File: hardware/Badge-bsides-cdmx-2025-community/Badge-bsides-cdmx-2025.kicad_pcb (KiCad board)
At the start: 2 copper layers, 50 x 110 mm, 30 parts, among them J1 SWDIO, J3 ADDON, J4 Conn_01x04_Pin, J5 I2C, J6 Conn_01x04_Pin, P6 USB_C_Plug_USB2.0, Q3 DMG3415U-7, SW11 ON, SW2 RESET, U1 PY32F030F28U6TR, U6 AP2112K-3.3

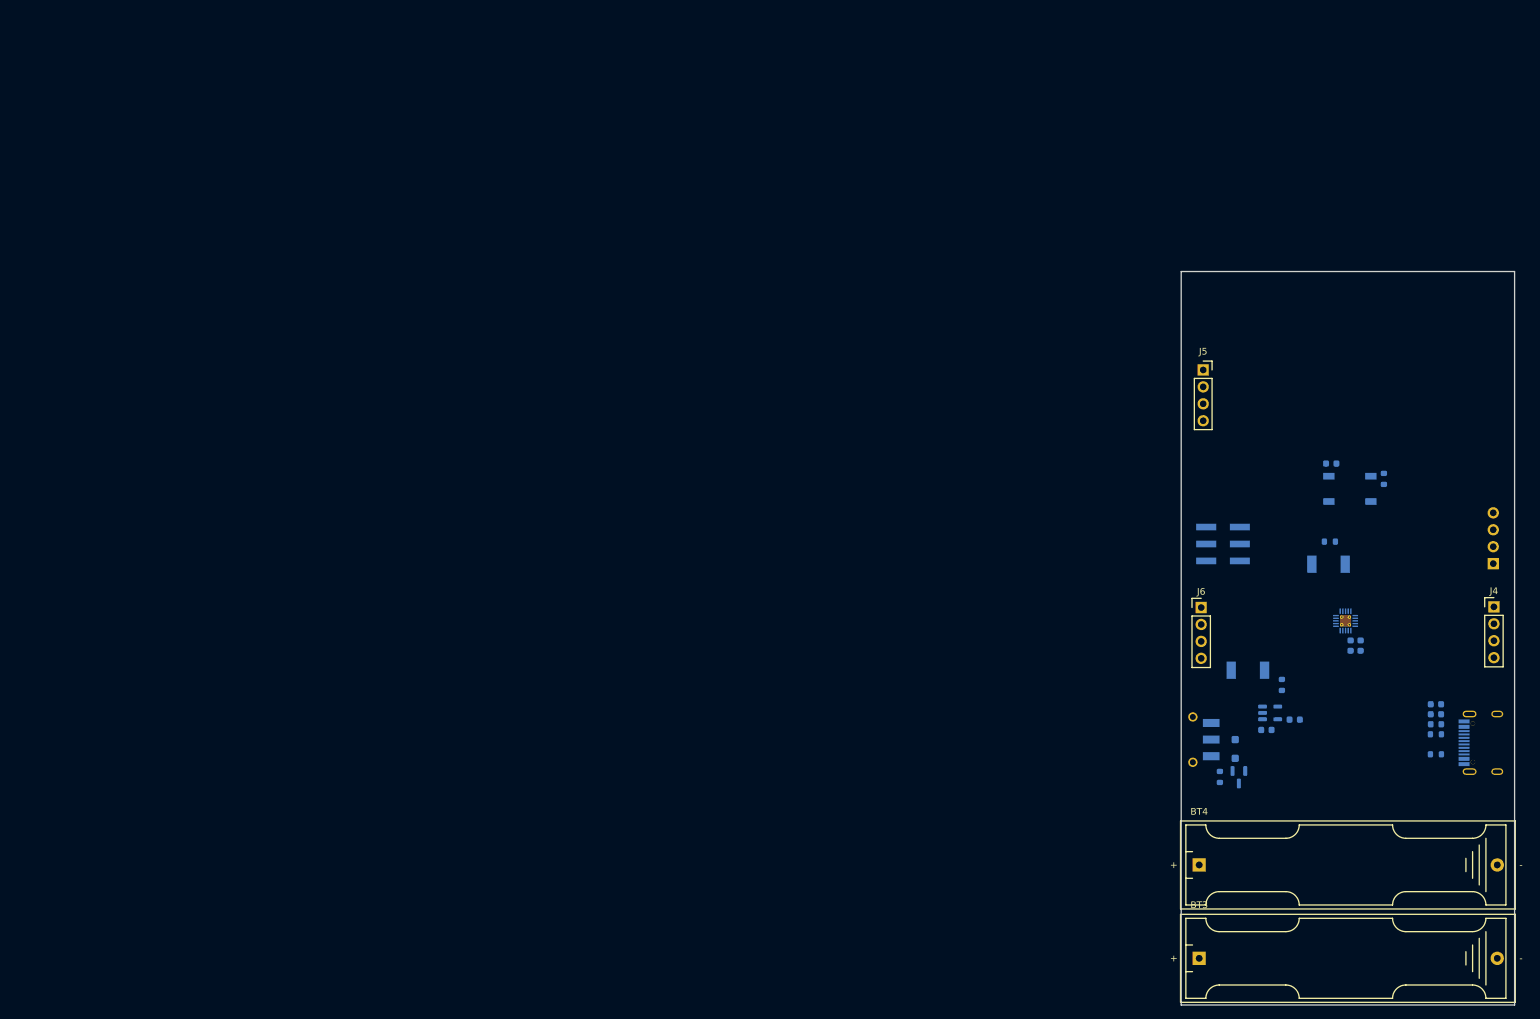
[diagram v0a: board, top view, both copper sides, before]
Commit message: feat(Hw):started_routing
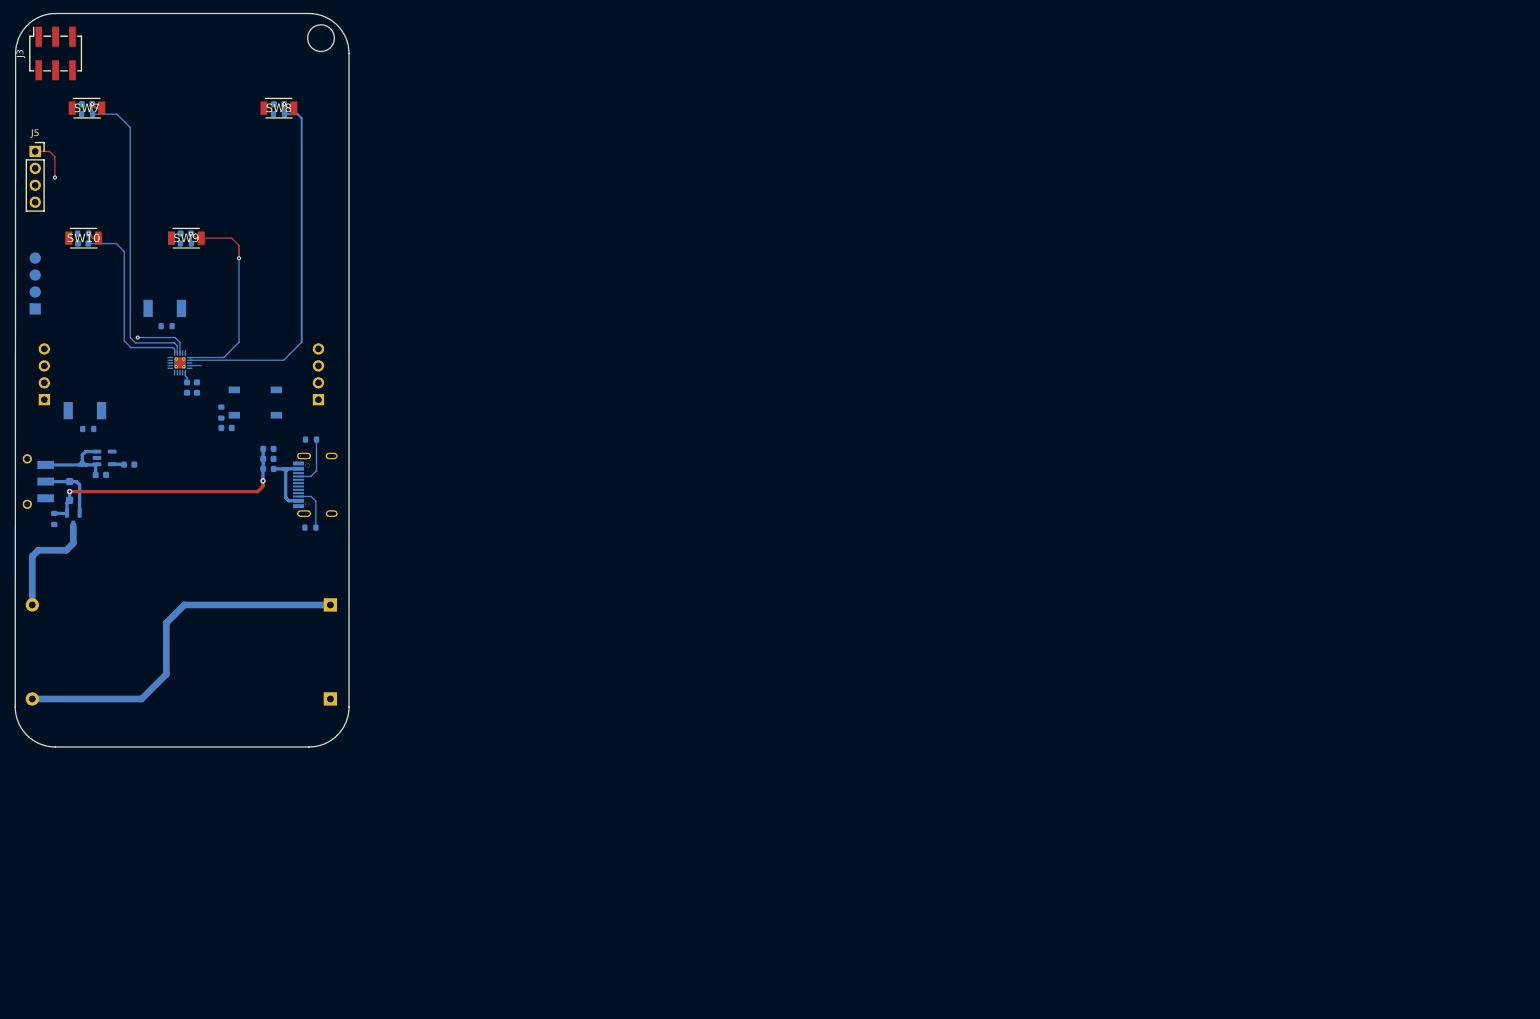
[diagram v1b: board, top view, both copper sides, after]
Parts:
- added C67: 10uF, Capacitor_SMD:C_0603_1608Metric, B.Cu at (-10.3, 13.9)
- added C68: 10uF, Capacitor_SMD:C_0603_1608Metric, B.Cu at (-24.3, 33.3)
- added C69: 10uF, Capacitor_SMD:C_0603_1608Metric, B.Cu at (-39.1, 13.9)
- added C70: 10uF, Capacitor_SMD:C_0603_1608Metric, B.Cu at (-39.7, 34.8)
- added R5: 10k, Resistor_SMD:R_0603_1608Metric, B.Cu at (-10.3, 15.4)
- added R6: 10k, Resistor_SMD:R_0603_1608Metric, B.Cu at (-24.3, 34.8)
- added R7: 10k, Resistor_SMD:R_0603_1608Metric, B.Cu at (-39.1, 15.4)
- added R8: 10k, Resistor_SMD:R_0603_1608Metric, B.Cu at (-39.7, 33.3)
- added SW10: SW_Push, Footprints:TS1088R02026, F.Cu at (-39.6, 34.0)
- added SW7: SW_Push, Footprints:TS1088R02026, F.Cu at (-39.1, 14.5)
- added SW8: SW_Push, Footprints:TS1088R02026, F.Cu at (-10.3, 14.5)
- added SW9: SW_Push, Footprints:TS1088R02026, F.Cu at (-24.2, 34.0)
- added kibuzzard-6841C014: G***, kibuzzard-6841C014, B.Cu at (-23.0, 89.0)
- BT3, BT4: moved to B.Cu
- J3: moved to F.Cu
- J4: footprint Connector_PinHeader_2.54mm:PinHeader_1x04_P2.54mm_Vertical -> Connector_PinHeader_2.54mm:PinHeader_1x04_P2.54mm_Horizontal; moved to B.Cu
- J6: footprint Connector_PinHeader_2.54mm:PinHeader_1x04_P2.54mm_Vertical -> Connector_PinSocket_2.54mm:PinSocket_1x04_P2.54mm_Horizontal; moved to B.Cu
- moved J1 222.0 mm to (-46.9, 44.6)
- moved J3 189.9 mm to (-43.8, 6.31), turned to 90 degrees
- moved D10 187.9 mm to (-39.4, 59.9)
- moved R11 187.0 mm to (-38.9, 62.6)
- moved C33 179.6 mm to (-11.9, 65.6)
- moved F3 179.2 mm to (-11.9, 68.6)
- moved D4 179.0 mm to (-41.7, 71.9)
- moved P6 179.0 mm to (-6.55, 71.0)
- moved Q3 179.0 mm to (-41.2, 76.1)
- moved R10 179.0 mm to (-44.0, 76.1)
- moved SW11 179.0 mm to (-46.3, 70.5)
- moved U1 179.0 mm to (-25.2, 52.7)
- moved J4 179.0 mm to (-4.38, 58.2)
- moved C10 178.9 mm to (-37.0, 69.5)
- moved C26 178.9 mm to (-32.8, 68.0)
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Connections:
- BT3 pad 2: +3.3V -> +BATT
- J3 pad 5: /GPIO1 -> /GPIO2
- J3 pad 6: /GPIO2 -> /GPIO1
- J4 pad 1: /RX -> GND
- J4 pad 2: /RX -> GND
- J4 pad 3: GND -> /RX
- J4 pad 4: GND -> /RX
- J6 pad 1: /TX -> GND
- J6 pad 2: /TX -> GND
- J6 pad 3: GND -> /TX
- J6 pad 4: GND -> /TX
- U1 pad 1: unconnected-(U1-PA5-Pad1) -> /BTTN2
- U1 pad 10: unconnected-(U1-PB6-Pad10) -> /LED1
- U1 pad 16: /GPIO2 -> /BTTN4
- U1 pad 17: /GPIO1 -> /BTTN3
- U1 pad 2: /LED1 -> /BTTN1
- U1 pad 20: unconnected-(U1-PA4-Pad20) -> /LED2
- U1 pad 3: /LED2 -> /GPIO1
- U1 pad 5: unconnected-(U1-PA12-Pad5) -> /GPIO2
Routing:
- net /BTTN1: track 0.00 -> 57.5 mm, vias 0 -> 1
- net Net-(BT3--): track 0.00 -> 55.1 mm
- net /BTTN3: track 0.00 -> 49.9 mm, vias 0 -> 1
- net VBUS: track 0.00 -> 40.2 mm, vias 0 -> 2
- net /BTTN2: track 0.00 -> 32.3 mm, vias 0 -> 2
- net /BTTN4: track 0.00 -> 31.3 mm, vias 0 -> 1
- net +BATT: track 0.00 -> 16.9 mm
- net Net-(SW11-A): track 0.00 -> 14.8 mm
- net Net-(F3-Pad1): track 0.00 -> 10.8 mm
- net Net-(D4-K): track 0.00 -> 9.51 mm
- net /TX: track 0.00 -> 8.26 mm, vias 0 -> 1
- net Net-(P6-CC): track 0.00 -> 7.73 mm
- net Net-(P6-VCONN): track 0.00 -> 6.86 mm
- net /SDA: track 0.00 -> 6.40 mm, vias 0 -> 1
- net +3V3: track 0.00 -> 1.80 mm
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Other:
- board size 50 x 110 mm -> 50.1 x 110 mm
